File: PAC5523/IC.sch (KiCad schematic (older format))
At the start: 18 parts, among them U11 ENCODER B, U2 ACT4088, U3 MAX3051, U5 ENCODER A, U6 RS485, U7 USBLC6-4, U8 USBLC6-4, U9 USBLC6-4

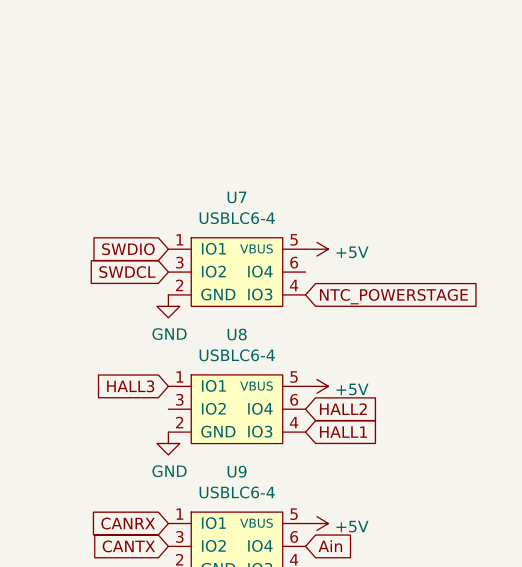
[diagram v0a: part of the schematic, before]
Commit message: placement almost done
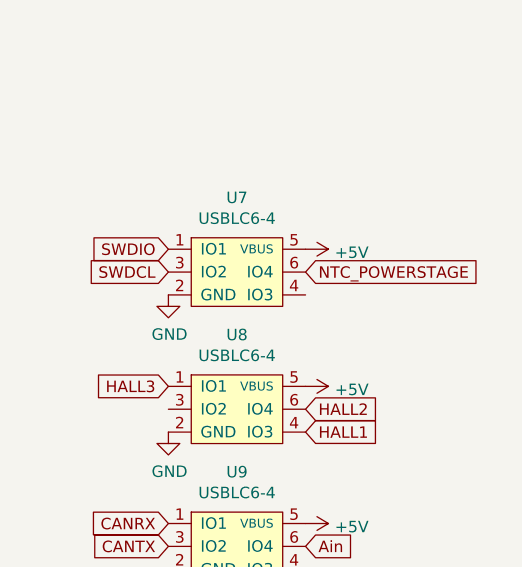
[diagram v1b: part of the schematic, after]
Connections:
- net NTC_POWERSTAGE: now also U7.6 (IO4); no longer U7.4 (IO3)
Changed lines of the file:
@@
 Text GLabel 8950 3250 0    50   Input ~ 0
 SWDIO
-Text GLabel 9550 3450 2    50   Input ~ 0
+Text GLabel 9550 3350 2    50   Input ~ 0
 NTC_POWERSTAGE
 Text GLabel 9550 4550 2    50   Input ~ 0
